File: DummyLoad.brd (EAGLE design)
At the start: 50.8 x 38.1 mm, 43 parts, among them IC1 LM358, J10 PINHD-1X1, J3 PINHD-1X1, J4 PINHD-1X1, J5 PINHD-1X1, J6 POWERJACK-OFFBRD, J7 PINHD-1X1, J8 PINHD-1X1, J9 PINHD-1X1, SW1 SWITCH-SPDT-OFFBRD, SW2 SWITCH-SPDT-OFFBRD, U1 LP2950

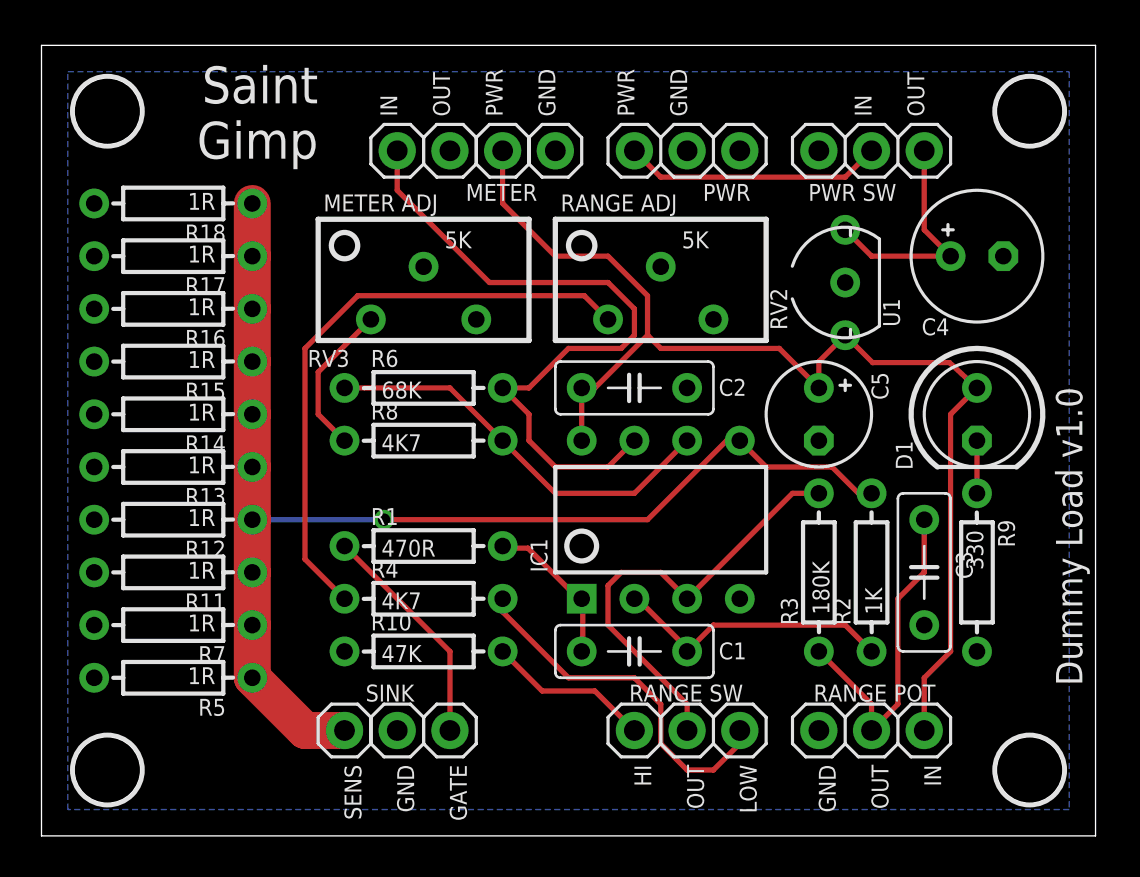
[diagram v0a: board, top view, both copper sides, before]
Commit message: Tweaked layout
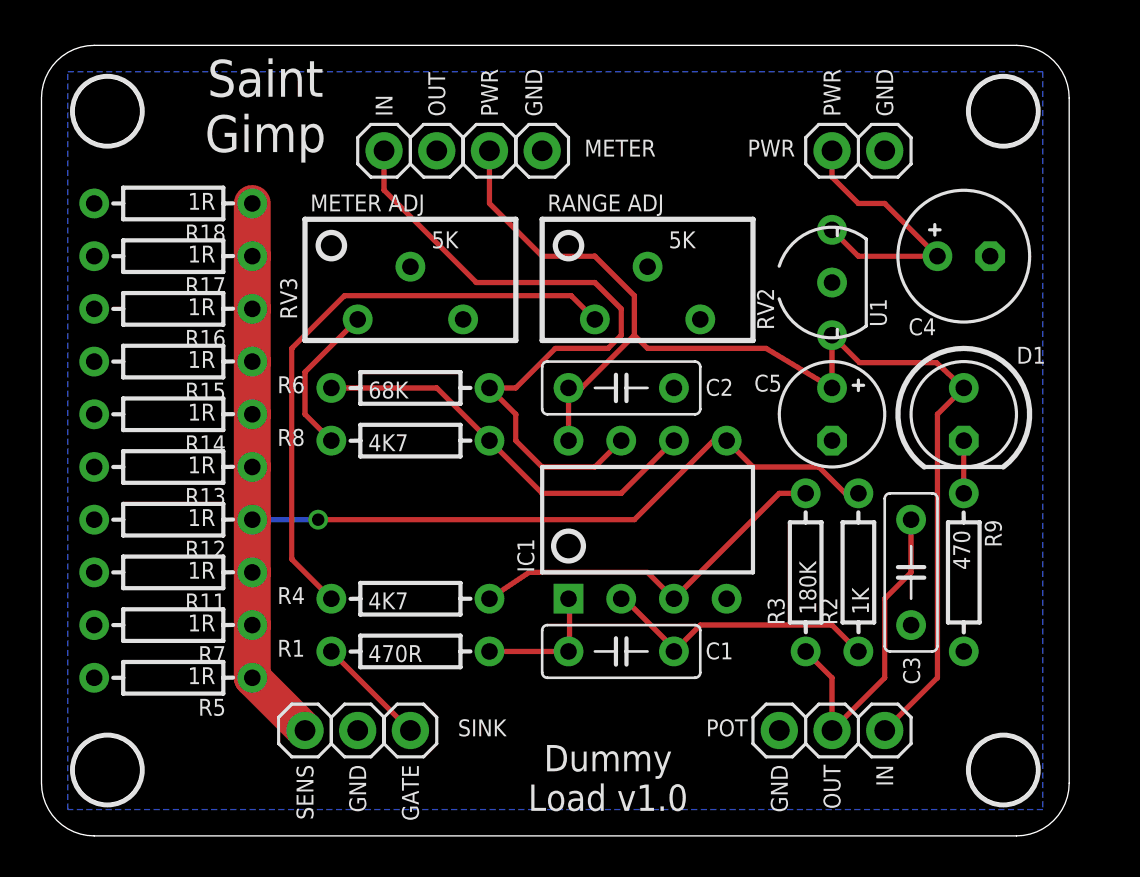
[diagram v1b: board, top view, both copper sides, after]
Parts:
- removed J6: POWERJACK-OFFBRD, SaintGimp:1X03
- removed R10: 47K, SaintGimp:AXIAL-7.5MM
- removed SW1, SW2: SWITCH-SPDT-OFFBRD, SaintGimp:1X03
- added J1: PINHD-1X2, SaintGimp:1X02
- D1: value LED -> LED-5MM
- IC1: value LM358 -> MCP6022
- R9: value 330 -> 470
- moved R1 5.12 mm to (17.8, 8.89)
- moved J4 1.91 mm to (12.7, 5.08)
- moved RV1 1.91 mm to (38.1, 5.08)
- moved J5 1.90 mm to (15.2, 5.08)
- moved J3 1.90 mm to (17.8, 5.08)
- moved U$3 1.27 mm to (46.4, 34.9)
- moved U$4 1.27 mm to (46.4, 3.17)
- moved C3 0.64 mm to (41.9, 12.7)
- moved R2 0.64 mm to (39.4, 12.7)
- moved R3 0.64 mm to (36.8, 12.7)
- moved J7 0.64 mm to (21.6, 33.0)
- moved J8 0.64 mm to (24.1, 33.0)
- moved C1 0.63 mm to (27.9, 8.89)
- moved C2 0.63 mm to (27.9, 21.6)
- moved C4 0.63 mm to (44.5, 27.9)
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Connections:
- removed net N$1: J6.1, SW2.2
- removed net N$10: R4.P$2, SW1.3
- removed net N$9: R10.P$2, SW1.1
- net GND: now also J1.2; no longer J6.2, J6.3, R10.P$1
- net N$13: now also R4.P$2; no longer SW1.2
- net N$3: now also J1.1; no longer SW2.3
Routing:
- net N$10: track 17.5 -> 0.00 mm
- net N$1: track 12.5 -> 0.00 mm
- net N$9: track 7.93 -> 0.00 mm
- net GATE: track 11.1 -> 5.39 mm
- net N$13: track 21.7 -> 18.3 mm
- net N$3: track 11.2 -> 13.5 mm
- net SENSE: track 60.4 -> 58.5 mm
- net N$2: track 7.52 -> 6.41 mm
- net +5V: track 57.3 -> 58.4 mm
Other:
- board size 50.8 x 38.1 mm -> 49.5 x 38.1 mm
- board text added: "POT"
- board text removed: "HI"
- board text removed: "LOW"
- board text removed: "PWR SW"
- board text removed: "RANGE POT"
- board text removed: "RANGE SW"
